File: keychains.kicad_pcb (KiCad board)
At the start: 2 copper layers, 106.4 x 105.3 mm, 166 parts

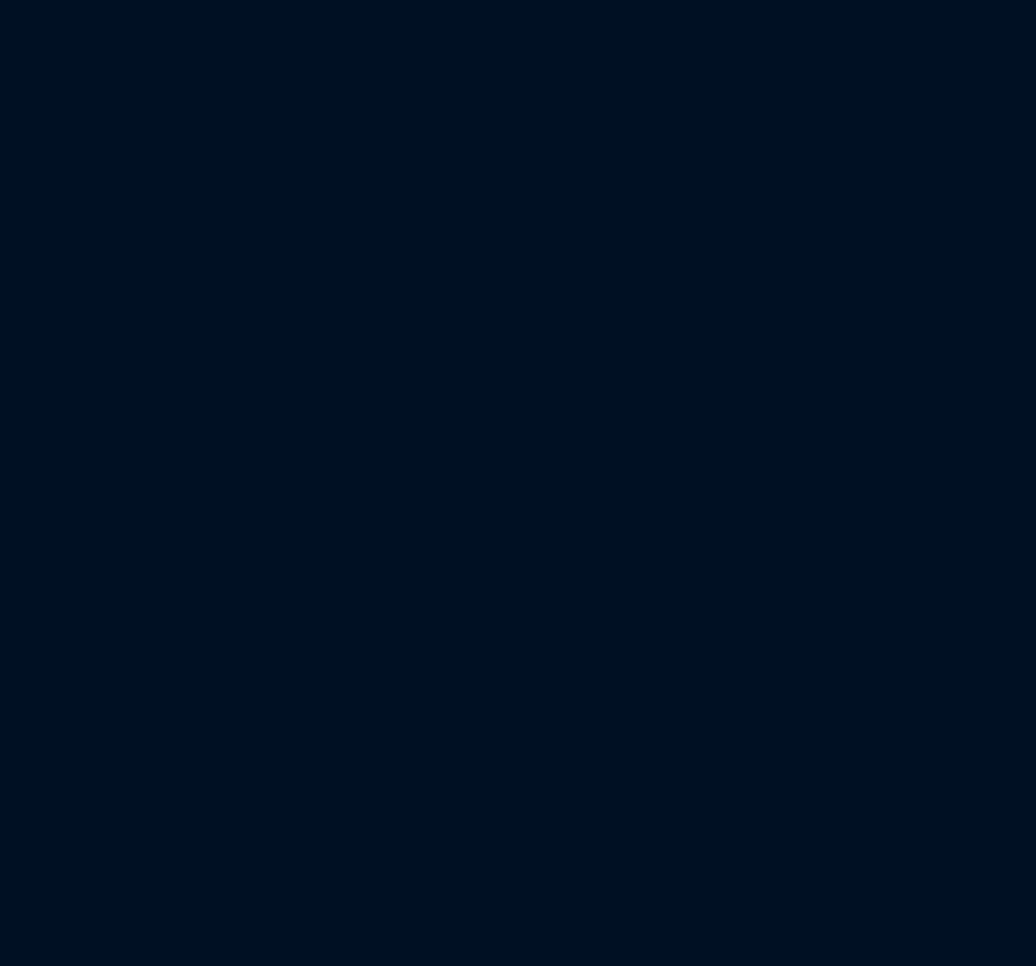
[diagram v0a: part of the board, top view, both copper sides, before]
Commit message: combined panel
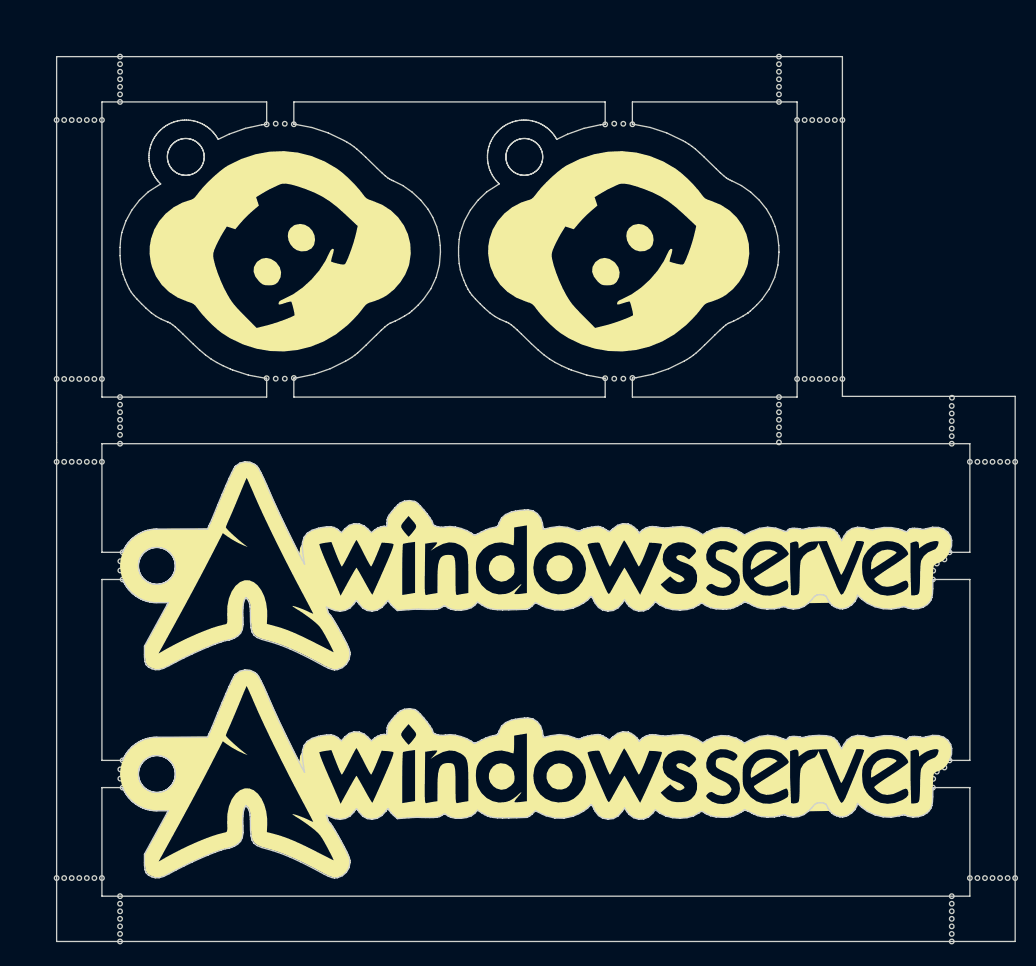
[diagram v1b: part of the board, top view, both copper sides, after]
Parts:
- added G***: LOGO, LOGO, F.Cu at (318.9, 112.6)
- added G*** (x2): LOGO, LOGO, F.Cu at (326.7, 54.9)
- added G*** (x2): LOGO, LOGO, F.Cu at (289.3, 54.9)
- added G***: LOGO, LOGO, F.Cu at (318.9, 89.7)
- added KiKit_MB_10_1: NPTH, NPTH, F.Cu at (264.7, 69.0)
- added KiKit_MB_10_1: NPTH, NPTH, F.Cu at (264.7, 124.1)
- added KiKit_MB_10_2: NPTH, NPTH, F.Cu at (265.5, 69.0)
- added KiKit_MB_10_2: NPTH, NPTH, F.Cu at (265.5, 124.1)
- added KiKit_MB_10_3: NPTH, NPTH, F.Cu at (266.3, 69.0)
- added KiKit_MB_10_3: NPTH, NPTH, F.Cu at (266.3, 124.1)
- added KiKit_MB_10_4: NPTH, NPTH, F.Cu at (267.2, 124.1)
- added KiKit_MB_10_4: NPTH, NPTH, F.Cu at (267.2, 69.0)
- added KiKit_MB_10_5: NPTH, NPTH, F.Cu at (268.0, 124.1)
- added KiKit_MB_10_5: NPTH, NPTH, F.Cu at (268.0, 69.0)
- added KiKit_MB_10_6: NPTH, NPTH, F.Cu at (268.8, 124.1)
- added KiKit_MB_10_6: NPTH, NPTH, F.Cu at (268.8, 69.0)
- added KiKit_MB_10_7: NPTH, NPTH, F.Cu at (269.7, 124.1)
- added KiKit_MB_10_7: NPTH, NPTH, F.Cu at (269.7, 69.0)
- added KiKit_MB_11_1: NPTH, NPTH, F.Cu at (346.4, 40.5)
- added KiKit_MB_11_1: NPTH, NPTH, F.Cu at (365.5, 78.2)
- added KiKit_MB_11_2: NPTH, NPTH, F.Cu at (366.3, 78.2)
- added KiKit_MB_11_2: NPTH, NPTH, F.Cu at (347.2, 40.5)
- added KiKit_MB_11_3: NPTH, NPTH, F.Cu at (348.1, 40.5)
- added KiKit_MB_11_3: NPTH, NPTH, F.Cu at (367.1, 78.2)
- added KiKit_MB_11_4: NPTH, NPTH, F.Cu at (368.0, 78.2)
- added KiKit_MB_11_4: NPTH, NPTH, F.Cu at (348.9, 40.5)
- added KiKit_MB_11_5: NPTH, NPTH, F.Cu at (368.8, 78.2)
- added KiKit_MB_11_5: NPTH, NPTH, F.Cu at (349.7, 40.5)
- added KiKit_MB_11_6: NPTH, NPTH, F.Cu at (350.6, 40.5)
- added KiKit_MB_11_6: NPTH, NPTH, F.Cu at (369.6, 78.2)
- added KiKit_MB_11_7: NPTH, NPTH, F.Cu at (351.4, 40.5)
- added KiKit_MB_11_7: NPTH, NPTH, F.Cu at (370.5, 78.2)
- added KiKit_MB_12_1: NPTH, NPTH, F.Cu at (346.4, 69.0)
- added KiKit_MB_12_1: NPTH, NPTH, F.Cu at (365.5, 124.1)
- added KiKit_MB_12_2: NPTH, NPTH, F.Cu at (366.3, 124.1)
- added KiKit_MB_12_2: NPTH, NPTH, F.Cu at (347.2, 69.0)
- added KiKit_MB_12_3: NPTH, NPTH, F.Cu at (348.1, 69.0)
- added KiKit_MB_12_3: NPTH, NPTH, F.Cu at (367.1, 124.1)
- added KiKit_MB_12_4: NPTH, NPTH, F.Cu at (368.0, 124.1)
- added KiKit_MB_12_4: NPTH, NPTH, F.Cu at (348.9, 69.0)
- added KiKit_MB_12_5: NPTH, NPTH, F.Cu at (349.7, 69.0)
- added KiKit_MB_12_5: NPTH, NPTH, F.Cu at (368.8, 124.1)
- added KiKit_MB_12_6: NPTH, NPTH, F.Cu at (350.6, 69.0)
- added KiKit_MB_12_6: NPTH, NPTH, F.Cu at (369.6, 124.1)
- added KiKit_MB_12_7: NPTH, NPTH, F.Cu at (351.4, 69.0)
- added KiKit_MB_12_7: NPTH, NPTH, F.Cu at (370.5, 124.1)
- added KiKit_MB_1_1: NPTH, NPTH, F.Cu at (271.9, 91.2)
- added KiKit_MB_1_1: NPTH, NPTH, F.Cu at (287.8, 40.9)
- added KiKit_MB_1_2: NPTH, NPTH, F.Cu at (288.8, 40.9)
- added KiKit_MB_1_2: NPTH, NPTH, F.Cu at (271.7, 90.2)
- added KiKit_MB_1_3: NPTH, NPTH, F.Cu at (289.8, 40.9)
- added KiKit_MB_1_3: NPTH, NPTH, F.Cu at (271.7, 89.1)
- added KiKit_MB_1_4: NPTH, NPTH, F.Cu at (271.9, 88.2)
- added KiKit_MB_1_4: NPTH, NPTH, F.Cu at (290.8, 40.9)
- added KiKit_MB_2_1: NPTH, NPTH, F.Cu at (363.2, 88.2)
- added KiKit_MB_2_1: NPTH, NPTH, F.Cu at (290.8, 68.9)
- added KiKit_MB_2_2: NPTH, NPTH, F.Cu at (289.8, 69.0)
- added KiKit_MB_2_2: NPTH, NPTH, F.Cu at (362.6, 88.9)
- added KiKit_MB_2_3: NPTH, NPTH, F.Cu at (361.8, 89.4)
- added KiKit_MB_2_3: NPTH, NPTH, F.Cu at (288.8, 69.0)
- added KiKit_MB_2_4: NPTH, NPTH, F.Cu at (361.4, 90.2)
- added KiKit_MB_2_4: NPTH, NPTH, F.Cu at (287.8, 68.9)
- added KiKit_MB_2_5: NPTH, NPTH, F.Cu at (361.4, 91.2)
- added KiKit_MB_3_1: NPTH, NPTH, F.Cu at (325.2, 40.9)
- added KiKit_MB_3_1: NPTH, NPTH, F.Cu at (271.9, 114.1)
- added KiKit_MB_3_2: NPTH, NPTH, F.Cu at (271.7, 113.1)
- added KiKit_MB_3_2: NPTH, NPTH, F.Cu at (326.2, 40.9)
- added KiKit_MB_3_3: NPTH, NPTH, F.Cu at (327.2, 40.9)
- added KiKit_MB_3_3: NPTH, NPTH, F.Cu at (271.7, 112.1)
- added KiKit_MB_3_4: NPTH, NPTH, F.Cu at (271.9, 111.1)
- added KiKit_MB_3_4: NPTH, NPTH, F.Cu at (328.2, 40.9)
- added KiKit_MB_4_1: NPTH, NPTH, F.Cu at (363.2, 111.1)
- added KiKit_MB_4_1: NPTH, NPTH, F.Cu at (328.2, 68.9)
- added KiKit_MB_4_2: NPTH, NPTH, F.Cu at (327.2, 69.0)
- added KiKit_MB_4_2: NPTH, NPTH, F.Cu at (362.6, 111.9)
- added KiKit_MB_4_3: NPTH, NPTH, F.Cu at (326.2, 69.0)
- added KiKit_MB_4_3: NPTH, NPTH, F.Cu at (361.8, 112.4)
- added KiKit_MB_4_4: NPTH, NPTH, F.Cu at (325.2, 68.9)
- added KiKit_MB_4_4: NPTH, NPTH, F.Cu at (361.4, 113.2)
- added KiKit_MB_4_5: NPTH, NPTH, F.Cu at (361.4, 114.1)
- added KiKit_MB_5_1: NPTH, NPTH, F.Cu at (271.7, 33.5)
- added KiKit_MB_5_2: NPTH, NPTH, F.Cu at (271.7, 34.3)
- added KiKit_MB_5_3: NPTH, NPTH, F.Cu at (271.7, 35.1)
- added KiKit_MB_5_4: NPTH, NPTH, F.Cu at (271.7, 36.0)
- added KiKit_MB_5_5: NPTH, NPTH, F.Cu at (271.7, 36.8)
- added KiKit_MB_5_6: NPTH, NPTH, F.Cu at (271.7, 37.6)
- added KiKit_MB_5_7: NPTH, NPTH, F.Cu at (271.7, 76.2)
- added KiKit_MB_5_7: NPTH, NPTH, F.Cu at (271.7, 38.5)
- added KiKit_MB_6_1: NPTH, NPTH, F.Cu at (344.4, 33.5)
- added KiKit_MB_6_1: NPTH, NPTH, F.Cu at (363.5, 71.1)
- added KiKit_MB_6_2: NPTH, NPTH, F.Cu at (344.4, 34.3)
- added KiKit_MB_6_2: NPTH, NPTH, F.Cu at (363.5, 72.0)
- added KiKit_MB_6_3: NPTH, NPTH, F.Cu at (363.5, 72.8)
- added KiKit_MB_6_3: NPTH, NPTH, F.Cu at (344.4, 35.1)
- added KiKit_MB_6_4: NPTH, NPTH, F.Cu at (363.5, 73.7)
- added KiKit_MB_6_4: NPTH, NPTH, F.Cu at (344.4, 36.0)
- added KiKit_MB_6_5: NPTH, NPTH, F.Cu at (363.5, 74.5)
- added KiKit_MB_6_5: NPTH, NPTH, F.Cu at (344.4, 36.8)
- added KiKit_MB_6_6: NPTH, NPTH, F.Cu at (363.5, 75.3)
- added KiKit_MB_6_6: NPTH, NPTH, F.Cu at (344.4, 37.6)
- added KiKit_MB_6_7: NPTH, NPTH, F.Cu at (363.5, 76.2)
- added KiKit_MB_6_7: NPTH, NPTH, F.Cu at (344.4, 38.5)
- added KiKit_MB_7_1: NPTH, NPTH, F.Cu at (271.7, 71.0)
- added KiKit_MB_7_1: NPTH, NPTH, F.Cu at (271.7, 126.1)
- added KiKit_MB_7_2: NPTH, NPTH, F.Cu at (271.7, 71.9)
- added KiKit_MB_7_2: NPTH, NPTH, F.Cu at (271.7, 126.9)
- added KiKit_MB_7_3: NPTH, NPTH, F.Cu at (271.7, 72.7)
- added KiKit_MB_7_3: NPTH, NPTH, F.Cu at (271.7, 127.8)
- added KiKit_MB_7_4: NPTH, NPTH, F.Cu at (271.7, 128.6)
- added KiKit_MB_7_4: NPTH, NPTH, F.Cu at (271.7, 73.5)
- added KiKit_MB_7_5: NPTH, NPTH, F.Cu at (271.7, 129.4)
- added KiKit_MB_7_5: NPTH, NPTH, F.Cu at (271.7, 74.4)
- added KiKit_MB_7_6: NPTH, NPTH, F.Cu at (271.7, 75.2)
- added KiKit_MB_7_6: NPTH, NPTH, F.Cu at (271.7, 130.3)
- added KiKit_MB_7_7: NPTH, NPTH, F.Cu at (271.7, 131.1)
- added KiKit_MB_8_1: NPTH, NPTH, F.Cu at (344.4, 71.0)
- added KiKit_MB_8_1: NPTH, NPTH, F.Cu at (363.5, 126.1)
- added KiKit_MB_8_2: NPTH, NPTH, F.Cu at (363.5, 126.9)
- added KiKit_MB_8_2: NPTH, NPTH, F.Cu at (344.4, 71.9)
- added KiKit_MB_8_3: NPTH, NPTH, F.Cu at (363.5, 127.8)
- added KiKit_MB_8_3: NPTH, NPTH, F.Cu at (344.4, 72.7)
- added KiKit_MB_8_4: NPTH, NPTH, F.Cu at (344.4, 73.5)
- added KiKit_MB_8_4: NPTH, NPTH, F.Cu at (363.5, 128.6)
- added KiKit_MB_8_5: NPTH, NPTH, F.Cu at (363.5, 129.4)
- added KiKit_MB_8_5: NPTH, NPTH, F.Cu at (344.4, 74.4)
- added KiKit_MB_8_6: NPTH, NPTH, F.Cu at (344.4, 75.2)
- added KiKit_MB_8_6: NPTH, NPTH, F.Cu at (363.5, 130.3)
- added KiKit_MB_8_7: NPTH, NPTH, F.Cu at (344.4, 76.0)
- added KiKit_MB_8_7: NPTH, NPTH, F.Cu at (363.5, 131.1)
- added KiKit_MB_9_1: NPTH, NPTH, F.Cu at (264.7, 78.2)
- added KiKit_MB_9_1: NPTH, NPTH, F.Cu at (264.7, 40.5)
- added KiKit_MB_9_2: NPTH, NPTH, F.Cu at (265.5, 40.5)
- added KiKit_MB_9_2: NPTH, NPTH, F.Cu at (265.5, 78.2)
- added KiKit_MB_9_3: NPTH, NPTH, F.Cu at (266.3, 40.5)
- added KiKit_MB_9_3: NPTH, NPTH, F.Cu at (266.3, 78.2)
- added KiKit_MB_9_4: NPTH, NPTH, F.Cu at (267.2, 40.5)
- added KiKit_MB_9_4: NPTH, NPTH, F.Cu at (267.2, 78.2)
- added KiKit_MB_9_5: NPTH, NPTH, F.Cu at (268.0, 40.5)
- added KiKit_MB_9_5: NPTH, NPTH, F.Cu at (268.0, 78.2)
- added KiKit_MB_9_6: NPTH, NPTH, F.Cu at (268.8, 40.5)
- added KiKit_MB_9_6: NPTH, NPTH, F.Cu at (268.8, 78.2)
- added KiKit_MB_9_7: NPTH, NPTH, F.Cu at (269.7, 40.5)
- added KiKit_MB_9_7: NPTH, NPTH, F.Cu at (269.7, 78.2)
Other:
- board size 106.4 x 105.3 mm -> 220.8 x 105.3 mm
